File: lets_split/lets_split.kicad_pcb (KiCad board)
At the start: 2 copper layers, 112 x 79 mm, 62 parts, among them J1 3PIN, J2 6PIN, J3 3PIN, SW1 SW_PUSH, SW10 SW_PUSH, SW11 SW_PUSH, SW12 SW_PUSH, SW13 SW_PUSH, SW14 SW_PUSH, SW15 SW_PUSH, SW16 SW_PUSH, SW17 SW_PUSH, SW18 SW_PUSH, SW19 SW_PUSH, SW2 SW_PUSH, SW21 SW_PUSH, SW22 SW_PUSH, SW23 SW_PUSH, SW3 SW_PUSH, SW4 SW_PUSH, SW5 SW_PUSH, SW6 SW_PUSH, SW7 SW_PUSH, SW8 SW_PUSH, SW9 SW_PUSH, U2 HOLE, U3 HOLE, U4 HOLE, U5 HOLE

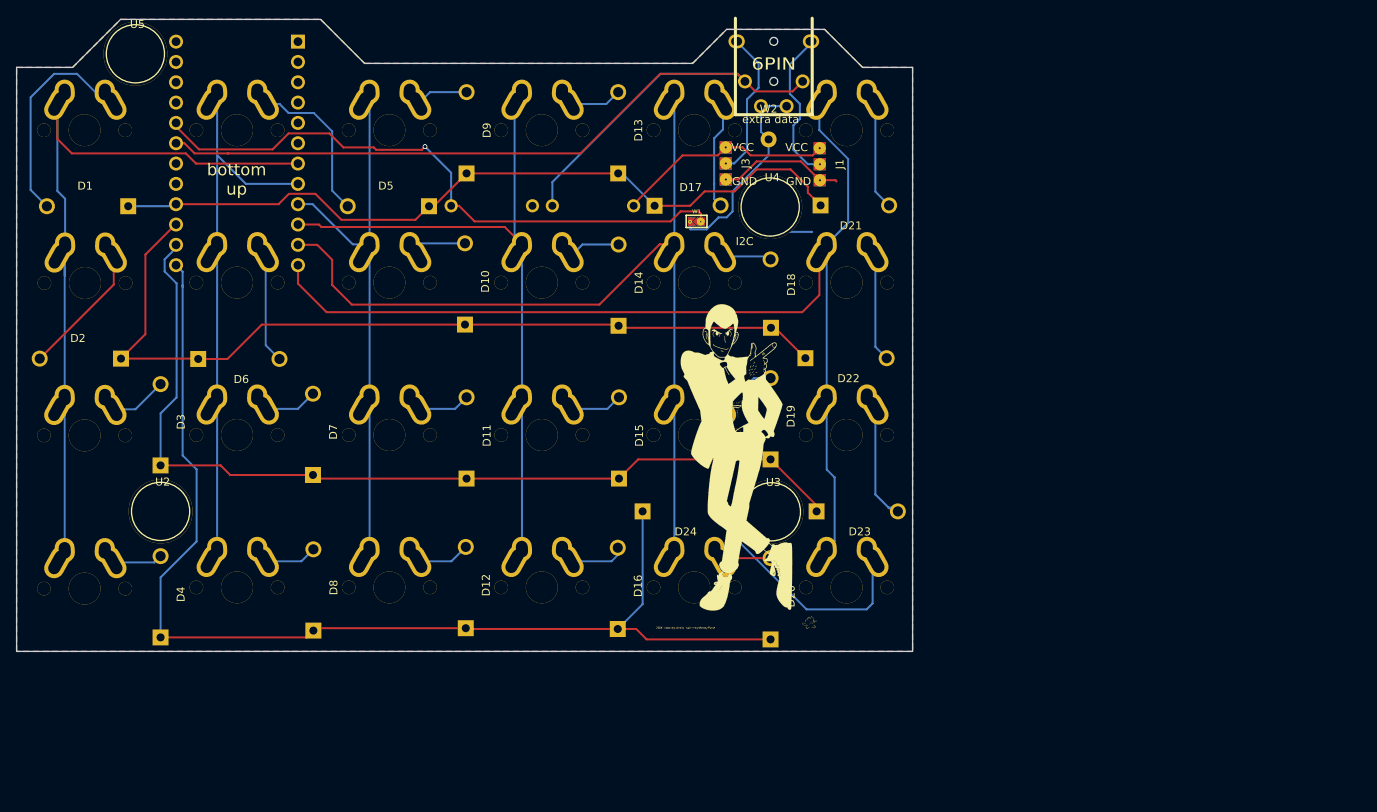
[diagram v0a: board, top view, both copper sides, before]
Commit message: Finished desing
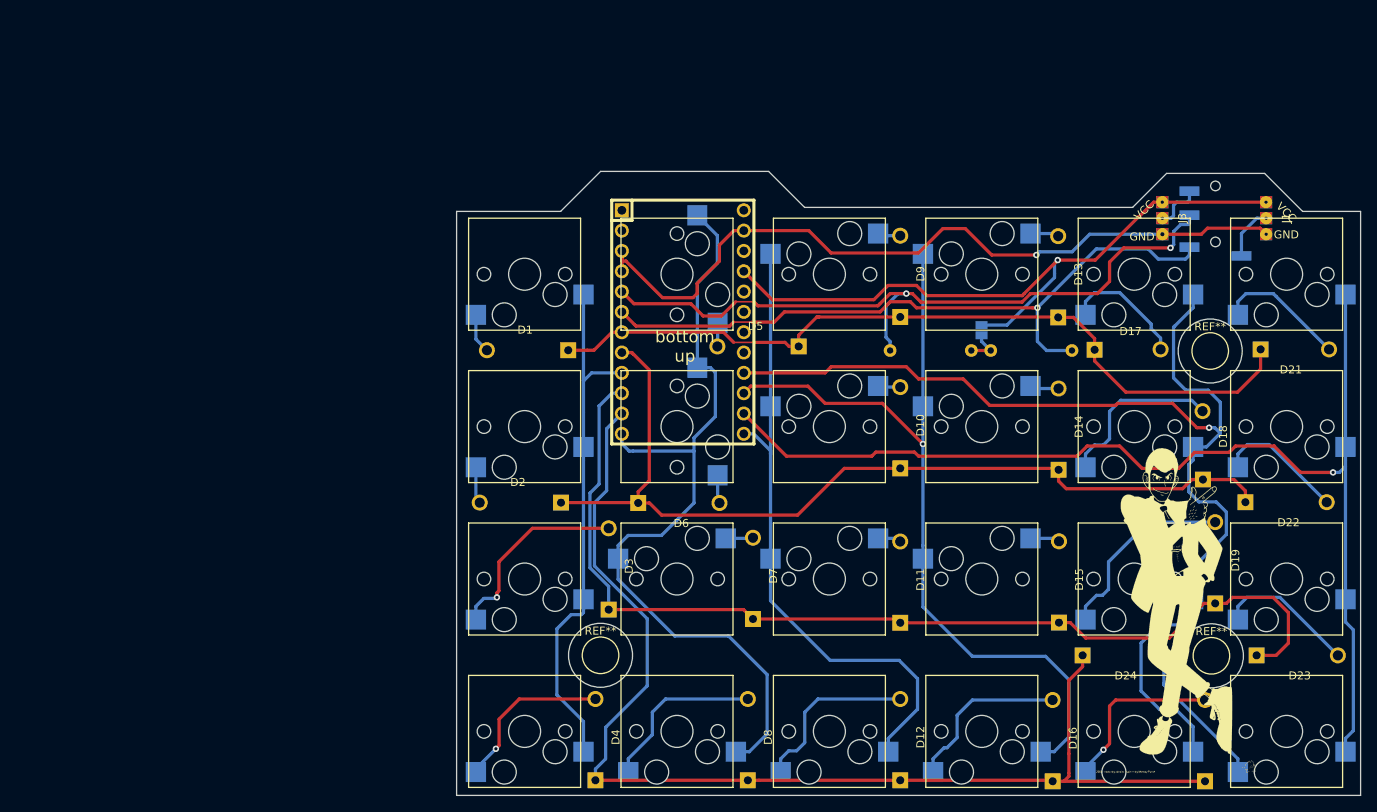
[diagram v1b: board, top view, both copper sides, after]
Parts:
- removed ? (x2): SW_PUSH, flipalps:MXALPS_FLIP
- removed U2, U3, U4, U5: HOLE, prettylib:HOLE
- removed W1: TEST, prettylib:JUMPER_SMD_2DUB
- removed W2: TEST_1P, Wire_Pads:SolderWirePad_single_2mmDrill
- added JP1: I2C / Serial, Jumpers:Solder-jumper-NO, B.Cu at (157.6, 71.8)
- added REF**: 1pin, Connect:1pin, F.Cu at (186.2, 74.5)
- added REF**: 1pin, Connect:1pin, F.Cu at (186.3, 112.5)
- added REF**: 1pin, Connect:1pin, F.Cu at (110.0, 112.5)
- added SW20: SW_PUSH, Kailh-socket, F.Cu at (119.5, 122.0)
- added SW24: SW_PUSH, Kailh-socket, F.Cu at (195.8, 122.0)
- J1, J3: footprint prettylib:jumper -> jumper-3pin-smd-dualside
- J2: value 6PIN -> CONN_01X04; footprint footprint:4pin35mmAudio -> Connectors:4ucon-20153; moved to B.Cu
- R1, R2: value R -> 4k7; footprint footprint:RESISTOR -> Resistors_ThroughHole:R_Axial_DIN0207_L6.3mm_D2.5mm_P10.16mm_Horizontal
- SW1, SW10, SW11, SW12, SW13, SW14, SW15, SW16, SW17, SW18, SW19, SW2, SW21, SW22, SW23, SW3, SW4, SW5, SW6, SW7, SW8, SW9: footprint flipalps:MXALPS_FLIP -> Kailh-socket
- U1: value (none) -> ArduinoProMicro; footprint footprint:TEENSY_2.0 -> plug-in-modules:ArduinoProMicro; moved to F.Cu
- moved SW6 131.2 mm to (195.8, 64.8), turned to 180 degrees
- moved SW4 118.8 mm to (157.7, 64.8)
- moved SW12 113.9 mm to (195.8, 83.9), turned to 180 degrees
- moved SW5 113.6 mm to (176.7, 64.8), turned to 180 degrees
- moved SW3 95.3 mm to (138.6, 64.8)
- moved SW11 93.1 mm to (176.7, 83.9), turned to 180 degrees
- moved SW18 82.8 mm to (195.8, 103.0), turned to 180 degrees
- moved SW17 78.6 mm to (176.7, 103.0), turned to 180 degrees
- moved SW10 76.2 mm to (157.7, 83.9)
- moved SW21 75.2 mm to (138.6, 122.0), turned to 180 degrees
- moved SW2 74.0 mm to (119.5, 64.8), turned to 270 degrees
- moved SW9 66.3 mm to (138.6, 83.9)
- moved R1 62.6 mm to (156.3, 74.4)
- moved J2 60.4 mm to (186.9, 57.3)
- moved U1 59.6 mm to (120.3, 70.8)
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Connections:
- J2 pad 2: data -> SCL/D3
- J2 pad 3: xtradata -> SDA
- R1 pad 1: VCC -> Net-(JP1-Pad2)
- R1 pad 2: Net-(R1-Pad2) -> SDA
- R2 pad 1: data -> Net-(JP1-Pad2)
- R2 pad 2: VCC -> SCL/D3
- SW10 pad 1: col2 -> col3
- SW10 pad 2: Net-(D10-Pad2) -> Net-(D14-Pad2)
- SW11 pad 1: col2 -> col4
- SW11 pad 2: Net-(D11-Pad2) -> Net-(D18-Pad2)
- SW12 pad 1: col2 -> col5
- SW12 pad 2: Net-(D12-Pad2) -> Net-(D22-Pad2)
- SW13 pad 1: col3 -> col0
- SW13 pad 2: Net-(D13-Pad2) -> Net-(D3-Pad2)
- SW14 pad 1: col3 -> col1
- SW14 pad 2: Net-(D14-Pad2) -> Net-(D7-Pad2)
- SW15 pad 1: col3 -> col2
- SW15 pad 2: Net-(D15-Pad2) -> Net-(D11-Pad2)
- SW16 pad 2: Net-(D16-Pad2) -> Net-(D15-Pad2)
- SW17 pad 2: Net-(D17-Pad2) -> Net-(D19-Pad2)
- SW18 pad 1: col4 -> col5
- SW18 pad 2: Net-(D18-Pad2) -> Net-(D23-Pad2)
- SW19 pad 1: col4 -> col0
- SW19 pad 2: Net-(D19-Pad2) -> Net-(D4-Pad2)
- SW2 pad 1: col0 -> col1
- SW2 pad 2: Net-(D2-Pad2) -> Net-(D5-Pad2)
- SW21 pad 1: col5 -> col2
- SW21 pad 2: Net-(D21-Pad2) -> Net-(D12-Pad2)
- SW22 pad 1: col5 -> col3
- SW22 pad 2: Net-(D22-Pad2) -> Net-(D16-Pad2)
- SW23 pad 1: col5 -> col4
- SW23 pad 2: Net-(D23-Pad2) -> Net-(D20-Pad2)
- SW3 pad 1: col0 -> col2
- SW3 pad 2: Net-(D3-Pad2) -> Net-(D9-Pad2)
- SW4 pad 1: col0 -> col3
- SW4 pad 2: Net-(D4-Pad2) -> Net-(D13-Pad2)
- SW5 pad 1: col1 -> col4
- SW5 pad 2: Net-(D5-Pad2) -> Net-(D17-Pad2)
- SW6 pad 1: col1 -> col5
- SW6 pad 2: Net-(D6-Pad2) -> Net-(D21-Pad2)
- SW7 pad 1: col1 -> col0
- SW7 pad 2: Net-(D7-Pad2) -> Net-(D2-Pad2)
- SW8 pad 2: Net-(D8-Pad2) -> Net-(D6-Pad2)
- SW9 pad 2: Net-(D9-Pad2) -> Net-(D10-Pad2)
- U1 pad 10: col3 -> row2
- U1 pad 11: col4 -> row3
- U1 pad 12: col5 -> col1
- U1 pad 18: row3 -> Net-(U1-Pad18)
- U1 pad 19: row2 -> Net-(U1-Pad19)
- U1 pad 2: GND -> Net-(U1-Pad2)
- U1 pad 20: row1 -> Net-(U1-Pad20)
- U1 pad 21: row0 -> VCC
- U1 pad 23: Net-(U1-Pad23) -> GND
- U1 pad 24: data -> Net-(U1-Pad24)
- U1 pad 3: Net-(U1-Pad3) -> GND
- U1 pad 4: VCC -> GND
- U1 pad 5: Net-(U1-Pad5) -> SDA
- U1 pad 6: Net-(U1-Pad6) -> SCL/D3
- U1 pad 7: col0 -> row0
- U1 pad 8: col1 -> row1
- U1 pad 9: col2 -> col0
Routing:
- net data: track 117.5 -> 0.00 mm
- net SDA: track 0.00 -> 90.7 mm, vias 0 -> 2
- net SCL/D3: track 0.00 -> 87.0 mm, vias 0 -> 1
- net GND: track 15.8 -> 97.1 mm, vias 0 -> 1
- net Net-(R1-Pad2): track 77.0 -> 0.00 mm, vias 1 -> 0
- net VCC: track 27.2 -> 86.8 mm, vias 0 -> 1
- net col1: track 68.7 -> 103.6 mm
- net col0: track 96.5 -> 65.9 mm
- net col4: track 112.3 -> 141.5 mm, vias 0 -> 1
- net xtradata: track 25.8 -> 0.00 mm
- net Net-(D1-Pad2): track 27.6 -> 4.99 mm
- net col3: track 85.0 -> 103.3 mm, vias 0 -> 1
- net Net-(D3-Pad2): track 7.20 -> 24.8 mm, vias 0 -> 1
- net Net-(D5-Pad2): track 19.9 -> 2.96 mm
- net Net-(D19-Pad2): track 7.54 -> 24.2 mm
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- removed copper zone on F.Cu, net GND
- removed copper zone on B.Cu, net VCC
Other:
- board size 112 x 79 mm -> 113 x 78 mm
- net class Default: clearance 0.2 -> 0.1524; trace_width 0.25 -> 0.1524; via_dia 0.6 -> 0.8
- rule trace_clearance: 0.2 -> 0.1524
- rule trace_min: 0.2 -> 0.1524
- board text removed: "I2C"
- board text removed: "extra data"
